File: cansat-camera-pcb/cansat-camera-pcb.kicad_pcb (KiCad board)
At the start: 8 copper layers, 50 x 50 mm, 63 parts, among them IC2 TLV74315PDBVR, J1 Conn_01x08_Pin, J2 Micro_SD_Card_Det2, J4 Conn_02x10_Odd_Even, J5 Conn_02x10_Odd_Even, J6 OV5640, SW2 SW_Push, U1 IS42S16800F-5TLI, U2 AP2112K-3.3, U4 STM32H743ZITx, U6 TLV74328PDBVR, Y1 24MHz

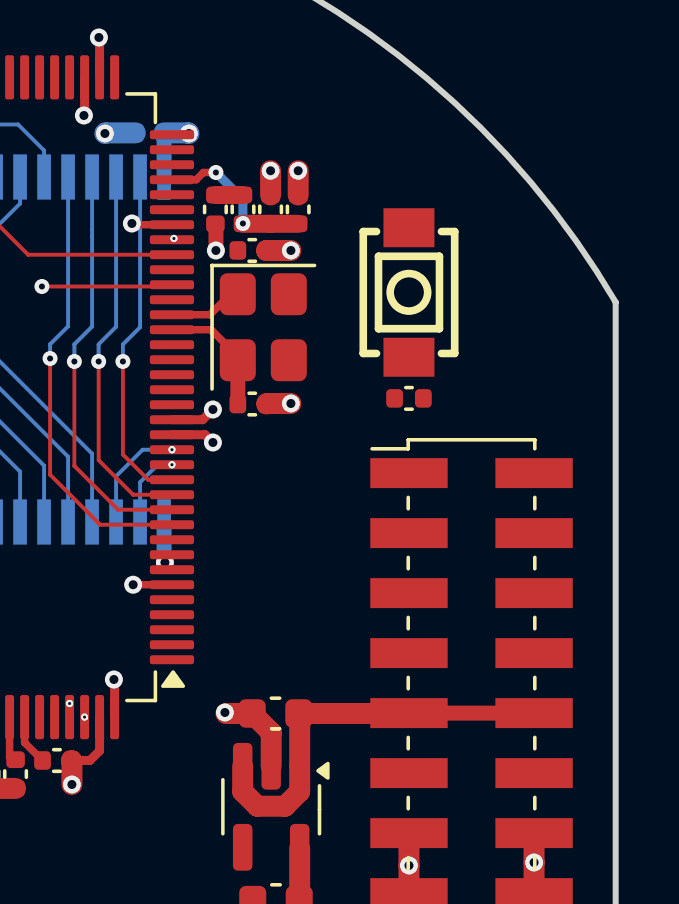
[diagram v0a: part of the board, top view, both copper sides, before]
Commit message: Routolás folytatása
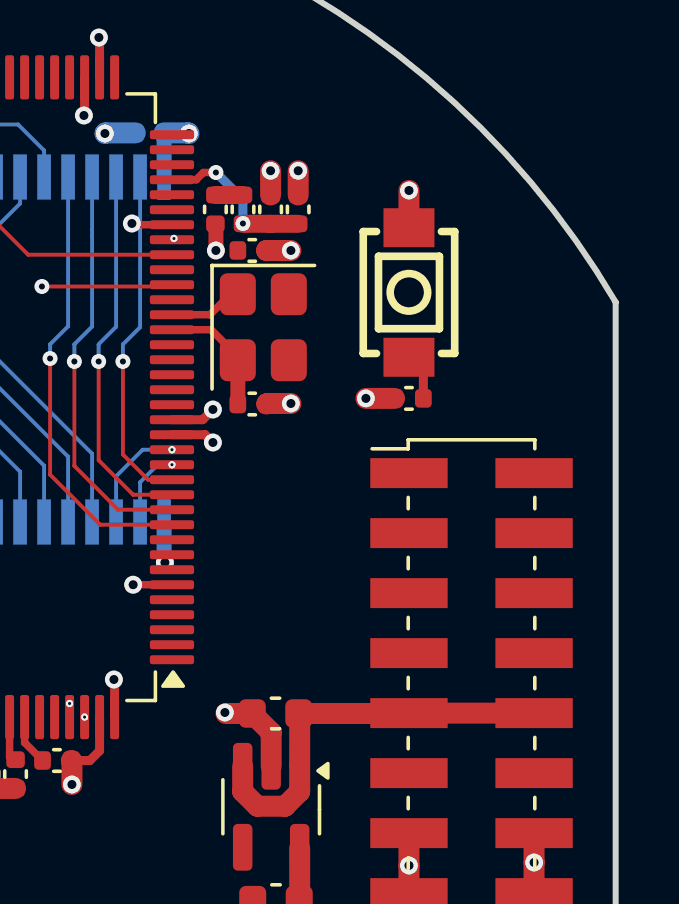
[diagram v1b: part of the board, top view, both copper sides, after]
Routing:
- net GND: track 61.3 -> 63.5 mm, vias 32 -> 34
- net /RST: track 0.00 -> 1.57 mm
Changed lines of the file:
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@@
+	)
+	(segment
+		(start 90.6 116.13)
+		(end 91.555 116.13)
+		(width 0.7)
+		(layer "F.Cu")
+		(net 1)
 	)
 	(segment
@@
 	)
 	(segment
+		(start 92.035 109.2)
+		(end 92.035 110.441)
+		(width 0.7)
+		(layer "F.Cu")
+		(net 1)
+	)
+	(segment
 		(start 61.092012 121.776)
 		(end 61.092012 120.807988)
@@
 	)
 	(via blind
+		(at 90.6 116.13)
+		(size 0.6)
+		(drill 0.3)
+		(layers "F.Cu" "In1.Cu")
+		(free yes)
+		(net 1)
+	)
+	(via blind
 		(at 60.2 110.7)
 		(size 0.6)
@@
 	(via blind
 		(at 86.827 133.9)
+		(size 0.6)
+		(drill 0.3)
+		(layers "F.Cu" "In1.Cu")
+		(free yes)
+		(net 1)
+	)
+	(via blind
+		(at 92.035 109.2)
 		(size 0.6)
 		(drill 0.3)
@@
 		(layer "F.Cu")
 		(net 2)
+	)
+	(segment
+		(start 92.515 116.13)
+		(end 92.515 115.239)
+		(width 0.3)
+		(layer "F.Cu")
+		(net 3)
+	)
+	(segment
+		(start 92.515 115.239)
+		(end 92.035 114.759)
+		(width 0.3)
+		(layer "F.Cu")
+		(net 3)
 	)
 	(segment
@@
 	)
 	(segment
+		(start 86.492 129.236544)
+		(end 86.492 128.393)
+		(width 0.7)
+		(layer "F.Cu")
+		(net 7)
+	)
+	(segment
+		(start 88.362 126.633)
+		(end 92.022 126.633)
+		(width 0.7)
+		(layer "F.Cu")
+		(net 7)
+	)
+	(segment
+		(start 87.904544 129.724)
+		(end 86.979456 129.724)
+		(width 0.7)
+		(layer "F.Cu")
+		(net 7)
+	)
+	(segment
+		(start 86.492 128.393)
+		(end 86.492 129.095122)
+		(width 0.5)
+		(layer "F.Cu")
+		(net 7)
+	)
+	(segment
 		(start 96.205 126.62)
 		(end 92.035 126.62)
-		(width 0.5)
+		(width 0.7)
 		(layer "F.Cu")
 		(net 7)
-	)
-	(segment
-		(start 86.492 129.236544)
-		(end 86.492 128.393)
-		(width 0.7)
-		(layer "F.Cu")
-		(net 7)
-	)
-	(segment
-		(start 88.362 126.633)
-		(end 92.022 126.633)
-		(width 0.7)
-		(layer "F.Cu")
-		(net 7)
-	)
-	(segment
-		(start 87.904544 129.724)
-		(end 86.979456 129.724)
-		(width 0.7)
-		(layer "F.Cu")
-		(net 7)
-	)
-	(segment
-		(start 86.492 128.393)
-		(end 86.492 129.095122)
-		(width 0.5)
-		(layer "F.Cu")
-		(net 7)

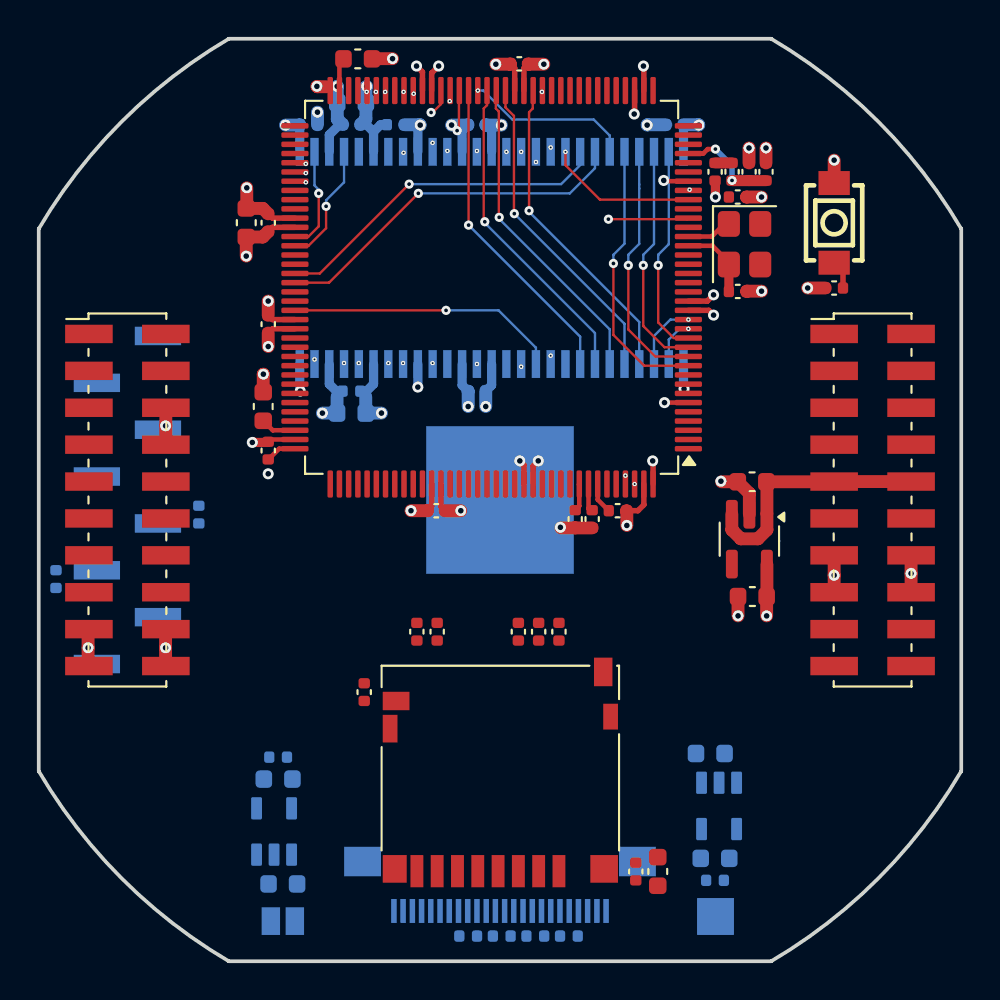
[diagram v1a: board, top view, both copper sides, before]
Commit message: Routolás folytatása
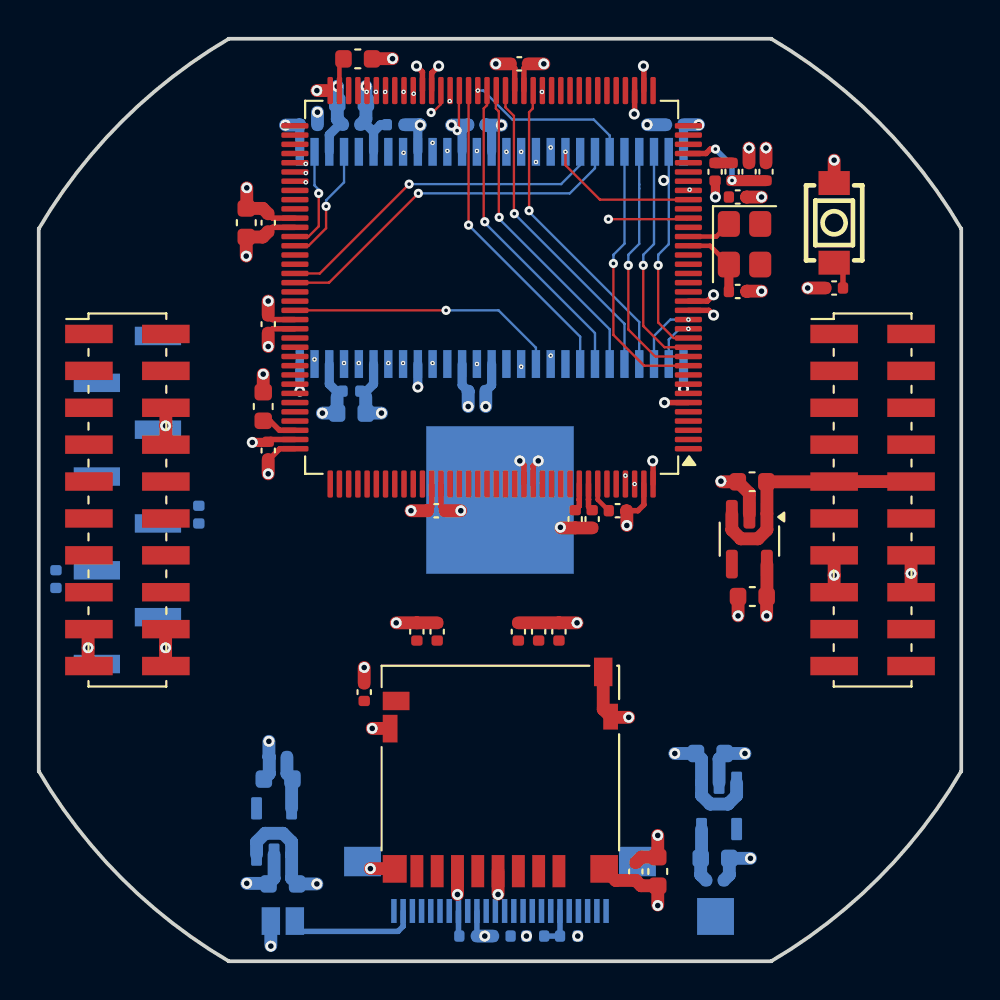
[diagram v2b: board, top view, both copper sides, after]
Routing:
- net GND: track 63.5 -> 87.7 mm, vias 34 -> 45
- net +3.3V: track 47.9 -> 71.9 mm, vias 23 -> 32
- net /camera/DATA1: track 0.00 -> 7.37 mm
- net /camera/2.8V_camera: track 0.00 -> 2.92 mm
- net /camera/1.5V_camera: track 0.00 -> 2.91 mm
- net /OV5640_RESET: track 0.00 -> 2.22 mm
- net /DCMI_PIXCLK: track 0.00 -> 1.38 mm
